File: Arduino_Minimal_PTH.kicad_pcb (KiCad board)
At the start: 2 copper layers, 27.9 x 45.7 mm, 22 parts, among them IC1 ATMEGA328P-PU, P1 I/O lo, P2 FTDI Basic, P3 A4 A5, P4 I/O hi, SW1 Reset, U1 L4931CZ50-AP, X1 CSTLS16M0X53-B0

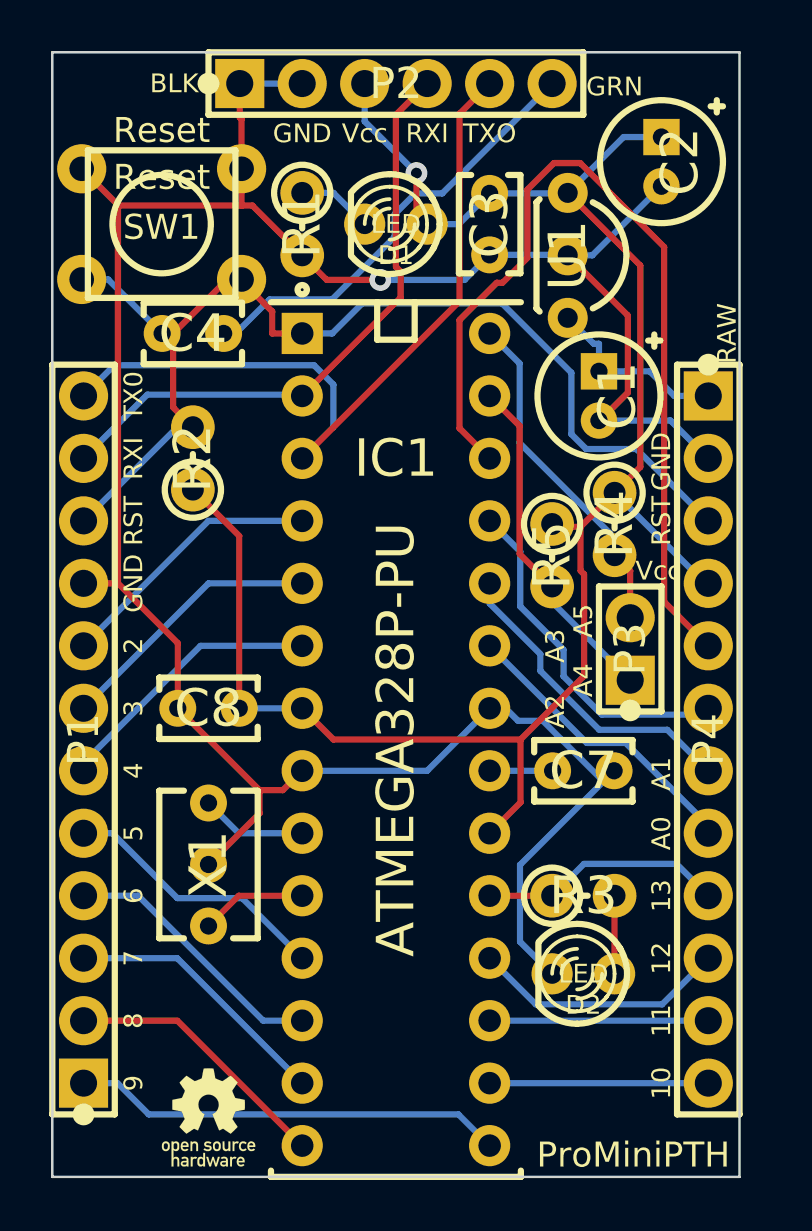
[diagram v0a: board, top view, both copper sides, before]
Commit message: Placed.
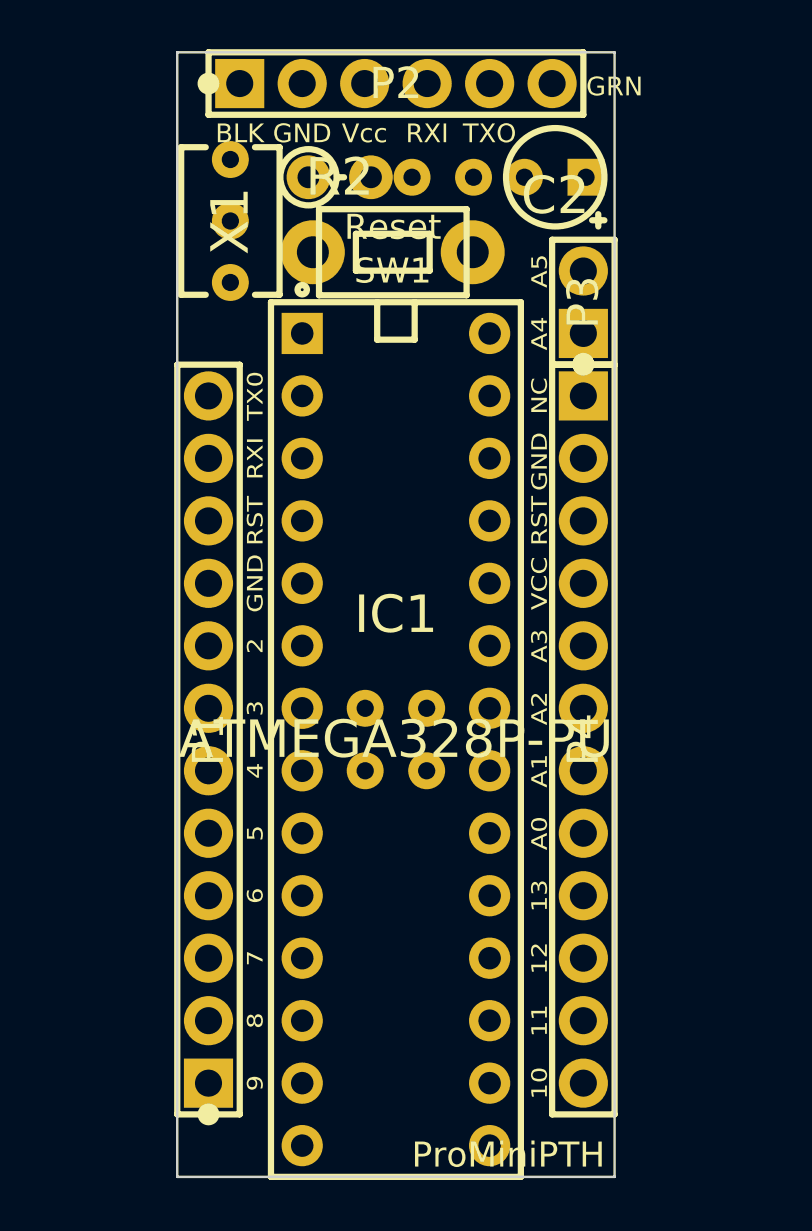
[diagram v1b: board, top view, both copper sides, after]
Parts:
- removed C1: 10u, mfk-CRP_5.0_2.0_0.5
- removed C3: 100n, mfk-C_4.0_2.5_2.5_0.5
- removed D1, D2: LED, LED-3MM
- removed R1: 10K, mfk-R_0.25W_RN55_vert
- removed R3: 330, mfk-R_0.25W_RN55_vert
- removed R4, R5: opt, mfk-R_0.25W_RN55_vert
- removed U1: L4931CZ50-AP, mfk-TO-92_f321
- removed VAL: REF, oshw-logo-150mil-FSilk
- C2: footprint mfk-CRP_5.0_2.0_0.5 -> mfk-CRP_4.0_2.5_0.5
- C4, C7, C8: moved to B.Cu
- SW1: footprint mfk-SW_PUSH_6MM -> mfk-SW_PUSH_6x3.5mm
- moved X1 26.2 mm to (129.2, 88.1)
- moved P3 14.2 mm to (143.5, 91.4)
- moved R2 12.9 mm to (133.6, 86.4), turned to 0 degrees
- moved C4 12.0 mm to (137.8, 86.4)
- moved SW1 9.47 mm to (135.8, 89.4)
- moved C7 7.62 mm to (135.9, 110.5), turned to 180 degrees
- moved C8 7.62 mm to (135.9, 108.0), turned to 0 degrees
- moved P1 5.08 mm to (128.3, 109.2)
- moved P4 5.08 mm to (143.5, 109.2)
- moved C2 4.36 mm to (142.4, 86.4), turned to 180 degrees
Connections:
- P4 pad 1: RAW -> (no net)
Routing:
- net GND: track 106.3 -> 0.00 mm, vias 1 -> 0
- net VCC: track 75.8 -> 0.00 mm, vias 1 -> 0
- net RESET: track 44.5 -> 0.00 mm
- net A3: track 37.1 -> 0.00 mm
- net TXO: track 32.9 -> 0.00 mm
- net RXI: track 24.9 -> 0.00 mm
- net DTR: track 18.1 -> 0.00 mm
- net D9: track 17.6 -> 0.00 mm
- net A2: track 14.2 -> 0.00 mm
- net A5: track 13.9 -> 0.00 mm
- net A4: track 13.9 -> 0.00 mm
- net A1: track 12.9 -> 0.00 mm
- net A0: track 12.2 -> 0.00 mm
- net D4: track 11.2 -> 0.00 mm
- net D6: track 11.0 -> 0.00 mm
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- removed copper zone on B.Cu, net GND
- removed copper zone on F.Cu, net GND
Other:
- board size 27.9 x 45.7 mm -> 17.8 x 45.7 mm
- board text added: "NC"
- board text added: "VCC"
- board text removed: "RAW"
- board text removed: "Reset"

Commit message: Routed
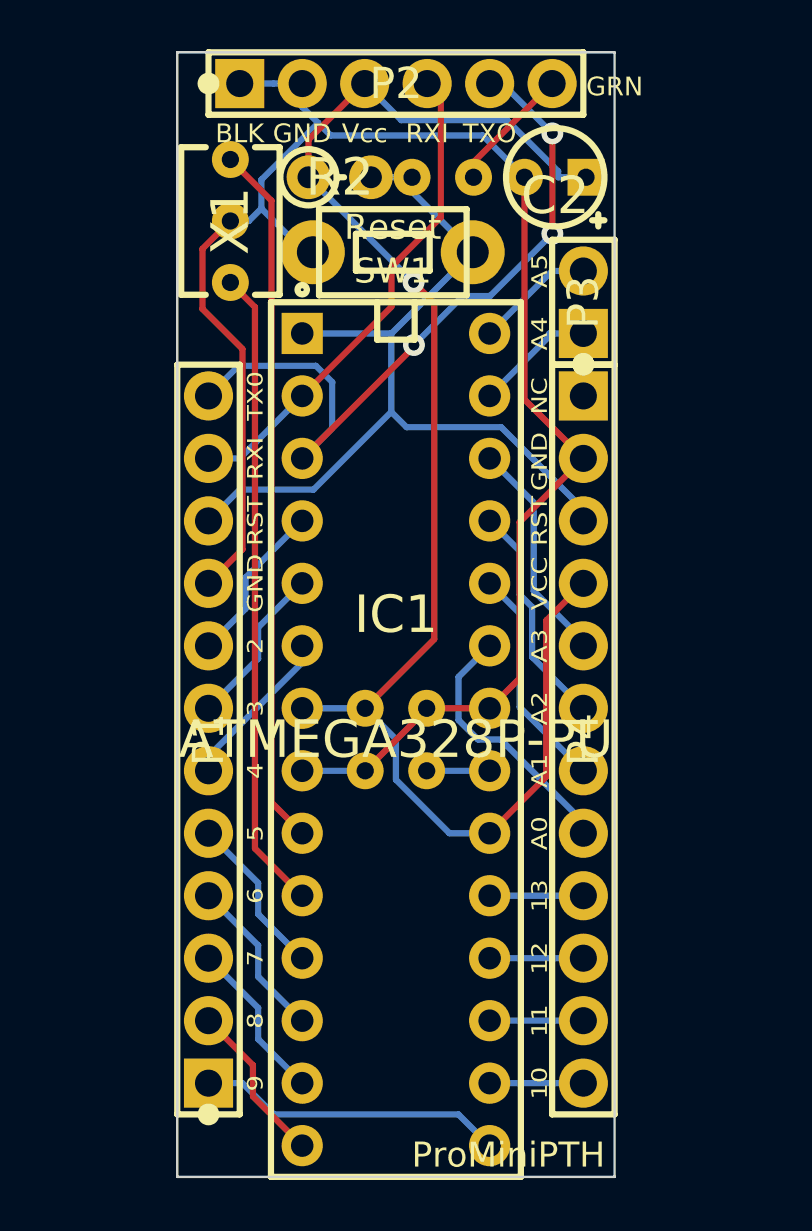
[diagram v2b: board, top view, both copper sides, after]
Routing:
- net GND: track 0.00 -> 71.8 mm
- net VCC: track 0.00 -> 62.8 mm, vias 0 -> 1
- net RESET: track 0.00 -> 36.4 mm
- net TXO: track 0.00 -> 30.9 mm, vias 0 -> 3
- net N-0000015: track 0.00 -> 28.6 mm
- net N-000005: track 0.00 -> 26.1 mm
- net RXI: track 0.00 -> 20.1 mm
- net D9: track 0.00 -> 12.5 mm
- net A0: track 0.00 -> 10.8 mm
- net A2: track 0.00 -> 9.20 mm
- net A1: track 0.00 -> 9.20 mm
- net A3: track 0.00 -> 9.20 mm
- net D6: track 0.00 -> 6.66 mm
- net D3: track 0.00 -> 6.66 mm
- net D8: track 0.00 -> 6.66 mm
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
